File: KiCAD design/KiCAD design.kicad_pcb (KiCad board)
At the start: 2 copper layers, 96 x 86 mm, 30 parts, among them J201 Conn_02x19_Odd_Even, J202 Conn_01x03_Female, J203 Conn_01x03_Female, J204 Conn_02x19_Odd_Even, J205 JST BATTERY, J206 JST SENS TOF 2, J208 JST SENS TOF 1, J401 Conn_02x06_Top_Bottom, U301 MCP1804T, U302 MIC5317, U401 ACS712xLCTR-20A

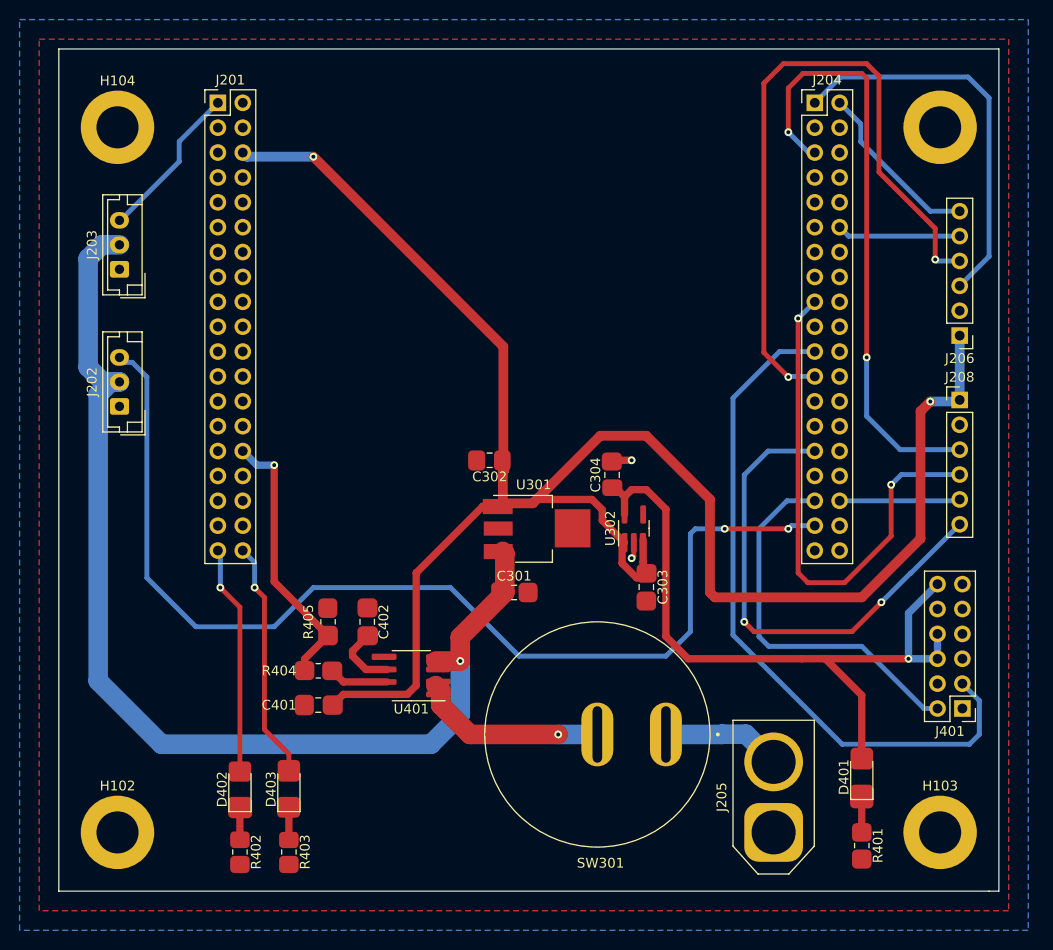
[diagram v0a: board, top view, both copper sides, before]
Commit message: Updated PCB and GRB files
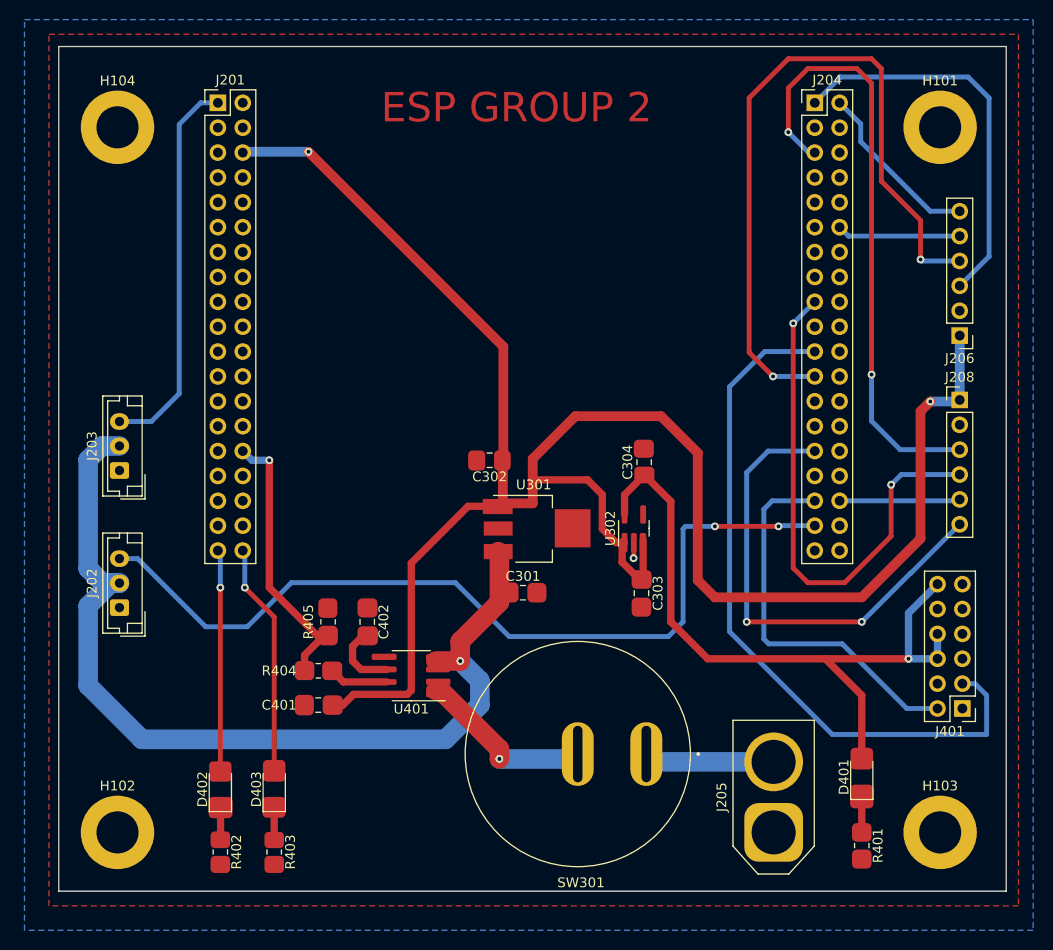
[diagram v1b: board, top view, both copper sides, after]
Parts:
- H101: moved to F.Cu
- moved J202 20.5 mm to (108.2, 109.0)
- moved J203 20.5 mm to (108.2, 95.0)
- moved C304 3.52 mm to (161.8, 94.2)
- moved SW301 2.83 mm to (155.0, 124.0)
- moved D402 2.00 mm to (118.5, 127.6)
- moved R402 2.00 mm to (118.5, 134.0)
- moved D403 1.50 mm to (124.0, 127.6)
- moved R403 1.50 mm to (124.0, 134.0)
- moved C301 0.90 mm to (149.4, 107.5)
- moved C303 0.80 mm to (161.5, 107.6)
- turned H101 to 0 degrees
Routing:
- net /CONNECTORS/USART_HD_BASE: track 16.2 -> 39.6 mm
- net /CONNECTORS/USART_HD_ARM: track 110.3 -> 88.3 mm
- net +12V: track 112.7 -> 95.4 mm
- net +5V: track 190.0 -> 198.6 mm
- net /CONNECTORS/TOF2_SCL: track 70.6 -> 74.5 mm
- net GND: track 4.08 -> 1.92 mm, vias 2 -> 1
- net /CONNECTORS/Bluetooth_TX: track 70.6 -> 72.8 mm
- net /CONNECTORS/BATT: track 12.2 -> 14.3 mm
- net /ON_BOARD_COMPONENTS/IP+: track 20.4 -> 19.1 mm
- net /CONNECTORS/LED2: track 23.9 -> 22.7 mm
- net /CONNECTORS/TOF1_DATA_READY: track 50.2 -> 49.0 mm
- net /CONNECTORS/LED1: track 24.9 -> 23.8 mm
- net /CONNECTORS/CURRENT_MEASURE: track 28.1 -> 28.9 mm
- net Net-(C402-Pad2): track 6.81 -> 7.38 mm
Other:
- board size 96 x 86 mm -> 96.8 x 86.2 mm
- board text added: "ESP GROUP 2"
